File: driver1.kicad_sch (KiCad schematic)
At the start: 91 parts, among them J1 FB CT, J2 24VDC INPUT, J3 MODE, J4 PHASE, J5 GDT, U1 L7809, U10 AOD609, U11 AOD609, U12 74AHC158, U2 MCP6567, U3 TLV3501AIDBV, U4 L7805, U5 IF-D95T, U6 74AHC14, U7 74AHC74, U8 74AHC1G08, U9 IX4340

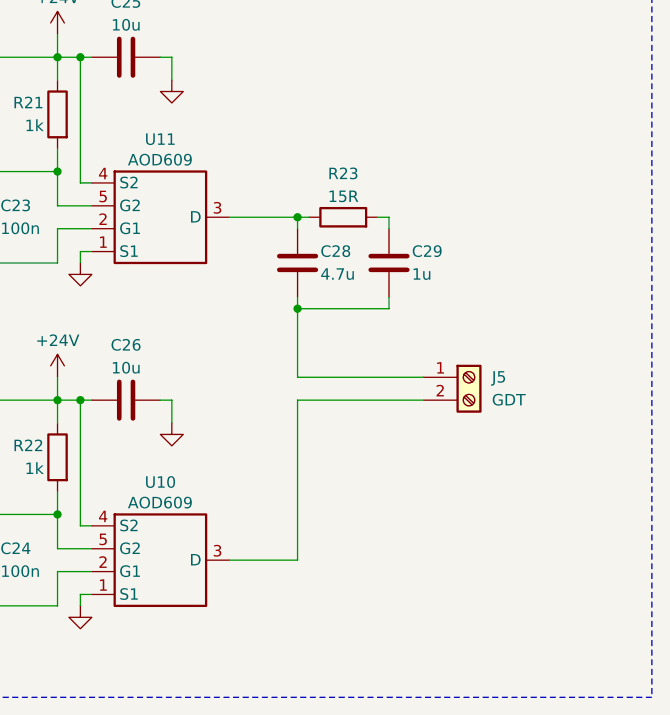
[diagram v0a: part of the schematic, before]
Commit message: almost done
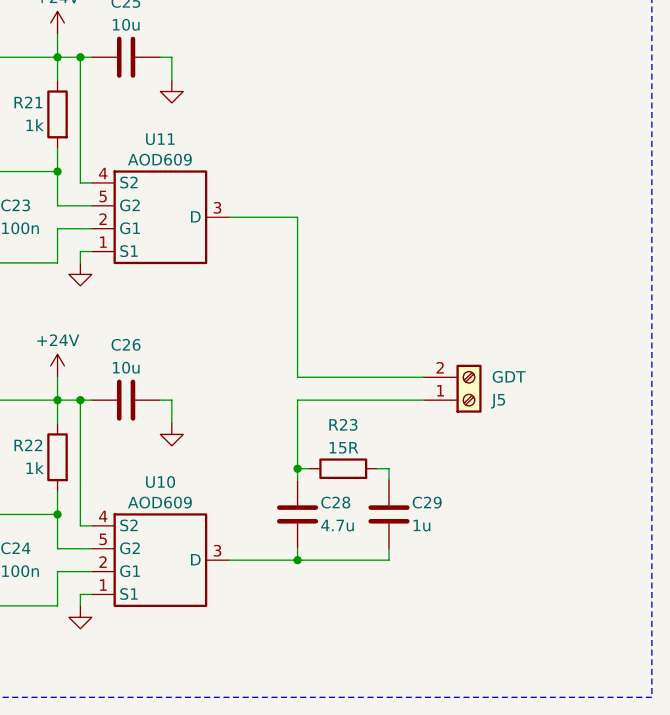
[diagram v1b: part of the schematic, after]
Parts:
- D5, D6, D7: footprint LED_THT:LED_D5.0mm -> LED_THT:LED_D3.0mm
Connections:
- net at C28.2, C29.2: now also U10.3 (D); no longer J5.1 (Pin_1)
- net at J5.2 (Pin_2): now also U11.3 (D); no longer U10.3 (D)
- net at C28.1, R23.1: now also J5.1 (Pin_1); no longer U11.3 (D)
